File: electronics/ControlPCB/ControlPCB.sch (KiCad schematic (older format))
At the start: 39 parts, among them CON1 12VINPUT, P1 Opto1, P2 Opto2, P3 Opto3, P4 Opto4, P5 Opto5, P6 Opto6, P7 Tool, U1 POLOLU_A4988, U2 POLOLU_A4988, U3 POLOLU_A4988, U4 POLOLU_A4988, U5 POLOLU_A4988, U6 POLOLU_A4988, U7 POLOLU_A4988

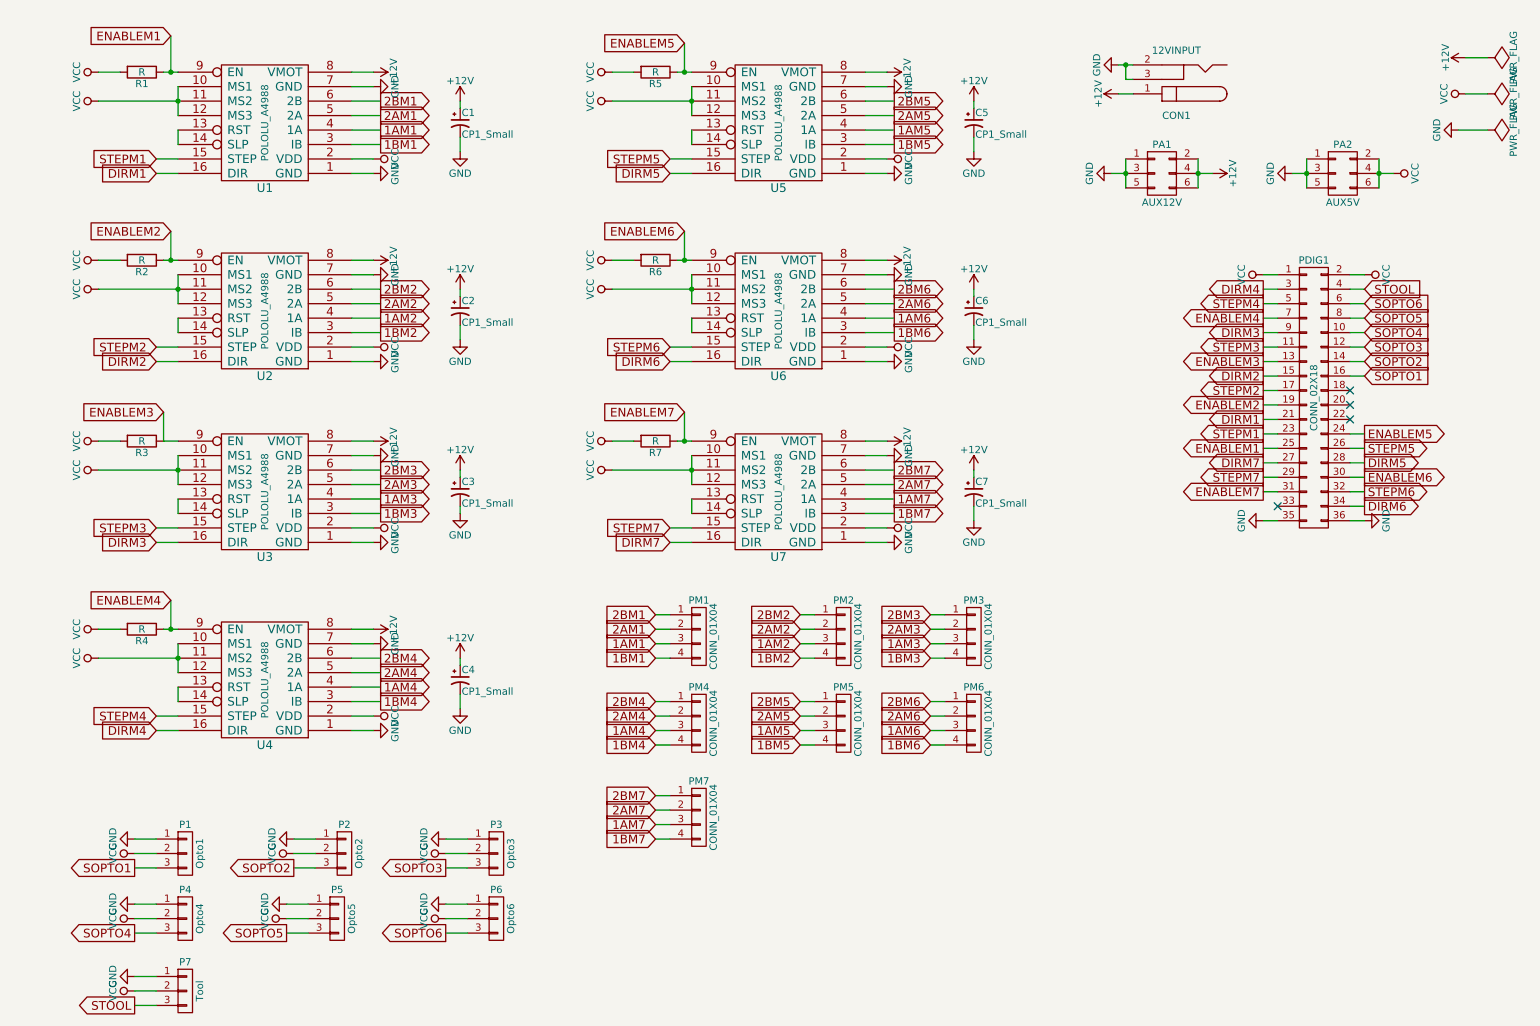
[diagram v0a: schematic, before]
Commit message: changes added
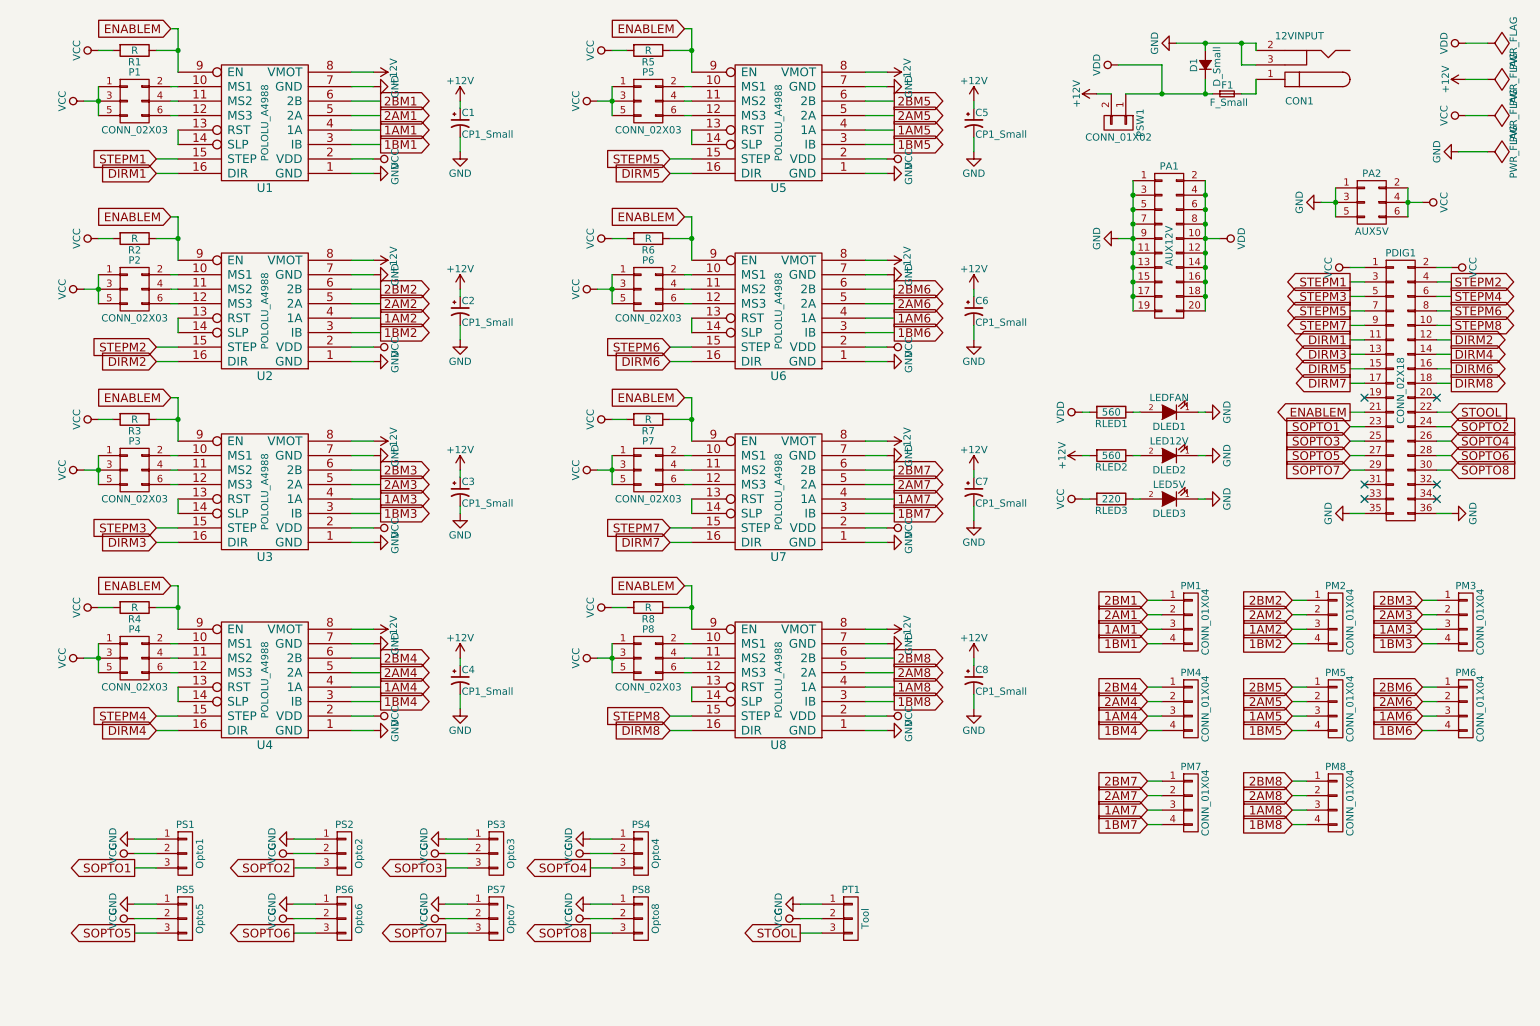
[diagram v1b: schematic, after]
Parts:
- removed PA1: AUX12V, Pin_Headers:Pin_Header_Straight_2x03, symbol CONN_02X03
- added C8: CP1_Small, Capacitors_ThroughHole:C_Radial_D6.3_L11.2_P2.5, symbol CP1_Small
- added D1: D_Small, symbol D_Small
- added DLED1: LEDFAN, symbol LED
- added DLED2: LED12V, symbol LED
- added DLED3: LED5V, symbol LED
- added F1: F_Small, symbol F_Small
- added P1, P2, P3, P4, P5, P6, P7, P8: CONN_02X03, symbol CONN_02X03
- added PA1: AUX12V, symbol CONN_02X10
- added PM8: CONN_01X04, Pin_Headers:Pin_Header_Straight_1x04, symbol CONN_01X04
- added PS7: Opto7, Pin_Headers:Pin_Header_Straight_1x03, symbol CONN_01X03
- added PS8: Opto8, Pin_Headers:Pin_Header_Straight_1x03, symbol CONN_01X03
- added PSW1: CONN_01X02, symbol CONN_01X02
- added R8: R, Resistors_ThroughHole:Resistor_Horizontal_RM7mm, symbol R
- added RLED1, RLED2: 560, symbol R
- added RLED3: 220, symbol R
- added U8: POLOLU_A4988, POL:POLA4988, symbol POLOLU_A4988
- renumbered P1 to PS1, P2 to PS2, P3 to PS3, P4 to PS4, P5 to PS5, P6 to PS6, P7 to PT1
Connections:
- net +12V: now also C8.1, PSW1.2 (P2), RLED2.2, U8.8 (VMOT); no longer CON1.1
- net DIRM1: now also PDIG1.11 (P11); no longer PDIG1.21 (P21)
- net DIRM2: now also PDIG1.12 (P12); no longer PDIG1.15 (P15)
- net DIRM3: now also PDIG1.13 (P13); no longer PDIG1.9 (P9)
- net DIRM4: now also PDIG1.14 (P14); no longer PDIG1.3 (P3)
- net DIRM5: now also PDIG1.15 (P15); no longer PDIG1.28 (P28)
- net DIRM6: now also PDIG1.16 (P16); no longer PDIG1.34 (P34)
- net DIRM7: now also PDIG1.17 (P17); no longer PDIG1.27 (P27)
- net GND: now also C8.2, D1.2 (A), DLED1.1 (K), DLED2.1 (K), DLED3.1 (K), PA1.1 (P1), PA1.11 (P11), PA1.13 (P13), PA1.15 (P15), PA1.17 (P17), PA1.19 (P19), PA1.3 (P3), PA1.5 (P5), PA1.7 (P7), PA1.9 (P9), PS7.1 (P1), PS8.1 (P1), U8.1 (GND), U8.7 (GND)
- net SOPTO1: now also PDIG1.23 (P23); no longer PDIG1.16 (P16)
- net SOPTO2: now also PDIG1.24 (P24); no longer PDIG1.14 (P14)
- net SOPTO3: now also PDIG1.25 (P25); no longer PDIG1.12 (P12)
- net SOPTO4: now also PDIG1.26 (P26); no longer PDIG1.10 (P10)
- net SOPTO5: now also PDIG1.27 (P27); no longer PDIG1.8 (P8)
- net SOPTO6: now also PDIG1.28 (P28); no longer PDIG1.6 (P6)
- net STEPM1: now also PDIG1.3 (P3); no longer PDIG1.23 (P23)
- net STEPM2: now also PDIG1.4 (P4); no longer PDIG1.17 (P17)
- net STEPM3: now also PDIG1.5 (P5); no longer PDIG1.11 (P11)
- net STEPM4: now also PDIG1.6 (P6); no longer PDIG1.5 (P5)
- net STEPM5: now also PDIG1.7 (P7); no longer PDIG1.26 (P26)
- net STEPM6: now also PDIG1.8 (P8); no longer PDIG1.32 (P32)
- net STEPM7: now also PDIG1.9 (P9); no longer PDIG1.29 (P29)
- net STOOL: now also PDIG1.22 (P22); no longer PDIG1.4 (P4)
- net VCC: now also P1.1 (P1), P1.3 (P3), P1.5 (P5), P2.1 (P1), P2.3 (P3), P2.5 (P5), P3.1 (P1), P3.3 (P3), P3.5 (P5), P4.1 (P1), P4.3 (P3), P4.5 (P5), P5.1 (P1), P5.3 (P3), P5.5 (P5), P6.1 (P1), P6.3 (P3), P6.5 (P5), P7.1 (P1), P7.3 (P3), P7.5 (P5), P8.1 (P1), P8.3 (P3), P8.5 (P5), PS7.2 (P2), PS8.2 (P2), R8.2, RLED3.2, U8.2 (VDD); no longer U1.10 (MS1), U1.11 (MS2), U1.12 (MS3), U2.10 (MS1), U2.11 (MS2), U2.12 (MS3), U3.10 (MS1), U3.11 (MS2), U3.12 (MS3), U4.10 (MS1), U4.11 (MS2), U4.12 (MS3), U5.10 (MS1), U5.11 (MS2), U5.12 (MS3), U6.10 (MS1), U6.11 (MS2), U6.12 (MS3), U7.10 (MS1), U7.11 (MS2), U7.12 (MS3)
- net DIRM8: now reaches PDIG1.18 (P18)
- net DIRM8: now also U8.16 (DIR)
- net ENABLEM1 renamed ENABLEM
- net ENABLEM: now also PDIG1.21 (P21), R2.1, R3.1, R4.1, R5.1, R6.1, R7.1, U2.9 (EN), U3.9 (EN), U4.9 (EN), U5.9 (EN), U6.9 (EN), U7.9 (EN), R8.1, U8.9 (EN); no longer PDIG1.25 (P25)
- removed net ENABLEM2: PDIG1.19 (P19), R2.1, U2.9 (EN)
- removed net ENABLEM3: PDIG1.13 (P13), R3.1, U3.9 (EN)
- removed net ENABLEM4: PDIG1.7 (P7), R4.1, U4.9 (EN)
- removed net ENABLEM5: PDIG1.24 (P24), R5.1, U5.9 (EN)
- removed net ENABLEM6: PDIG1.30 (P30), R6.1, U6.9 (EN)
- removed net ENABLEM7: PDIG1.31 (P31), R7.1, U7.9 (EN)
- new net: P1.2 (P2), U1.10 (MS1)
- new net: P1.4 (P4), U1.11 (MS2)
- new net: P1.6 (P6), U1.12 (MS3)
- new net: P2.2 (P2), U2.10 (MS1)
- new net: P2.4 (P4), U2.11 (MS2)
- new net: P2.6 (P6), U2.12 (MS3)
- new net: P3.2 (P2), U3.10 (MS1)
- new net: P3.4 (P4), U3.11 (MS2)
- new net: P3.6 (P6), U3.12 (MS3)
- new net: P4.2 (P2), U4.10 (MS1)
- new net: P4.4 (P4), U4.11 (MS2)
- new net: P4.6 (P6), U4.12 (MS3)
- new net: P5.2 (P2), U5.10 (MS1)
- new net: P5.4 (P4), U5.11 (MS2)
- new net: P5.6 (P6), U5.12 (MS3)
- new net: P6.2 (P2), U6.10 (MS1)
- new net: P6.4 (P4), U6.11 (MS2)
- new net: P6.6 (P6), U6.12 (MS3)
- new net: P7.2 (P2), U7.10 (MS1)
- new net: P7.4 (P4), U7.11 (MS2)
- new net: P7.6 (P6), U7.12 (MS3)
- new net: CON1.1, F1.2
- new net: P8.2 (P2), U8.10 (MS1)
- new net: P8.4 (P4), U8.11 (MS2)
- new net: P8.6 (P6), U8.12 (MS3)
- new net: U8.13 (RST), U8.14 (SLP)
- new net: DLED1.2 (A), RLED1.1
- new net: DLED2.2 (A), RLED2.1
- new net: DLED3.2 (A), RLED3.1
- new net 1AM8: PM8.3 (P3), U8.4 (1A)
- new net 1BM8: PM8.4 (P4), U8.3 (IB)
- new net 2AM8: PM8.2 (P2), U8.5 (2A)
- new net 2BM8: PM8.1 (P1), U8.6 (2B)
- new net SOPTO7: PDIG1.29 (P29), PS7.3 (P3)
- new net SOPTO8: PDIG1.30 (P30), PS8.3 (P3)
- new net STEPM8: PDIG1.10 (P10), U8.15 (STEP)
- new net VDD: D1.1 (K), F1.1, PA1.10 (P10), PA1.12 (P12), PA1.14 (P14), PA1.16 (P16), PA1.18 (P18), PA1.2 (P2), PA1.20 (P20), PA1.4 (P4), PA1.6 (P6), PA1.8 (P8), PSW1.1 (P1), RLED1.2
- no-connect marks 4 -> 6
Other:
- moved on the sheet: CON1, PA2, PDIG1, PM1, PM2, PM3, PM4, PM5, PM6, PM7, PS4, PS5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

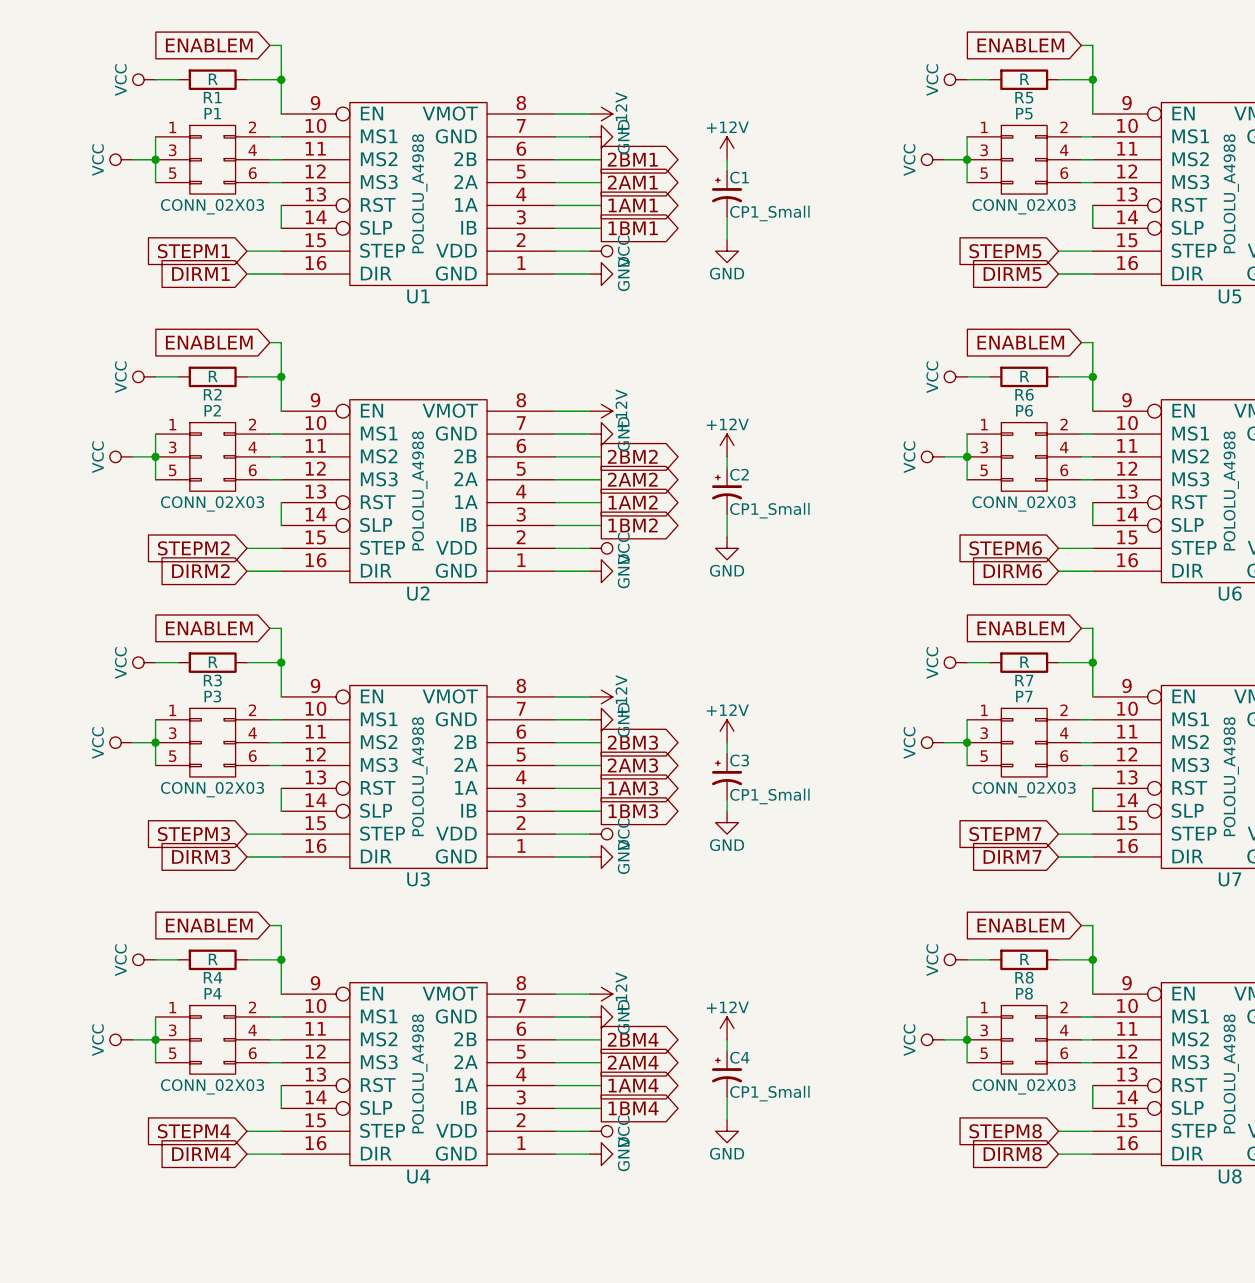
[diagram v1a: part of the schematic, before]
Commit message: PCB update
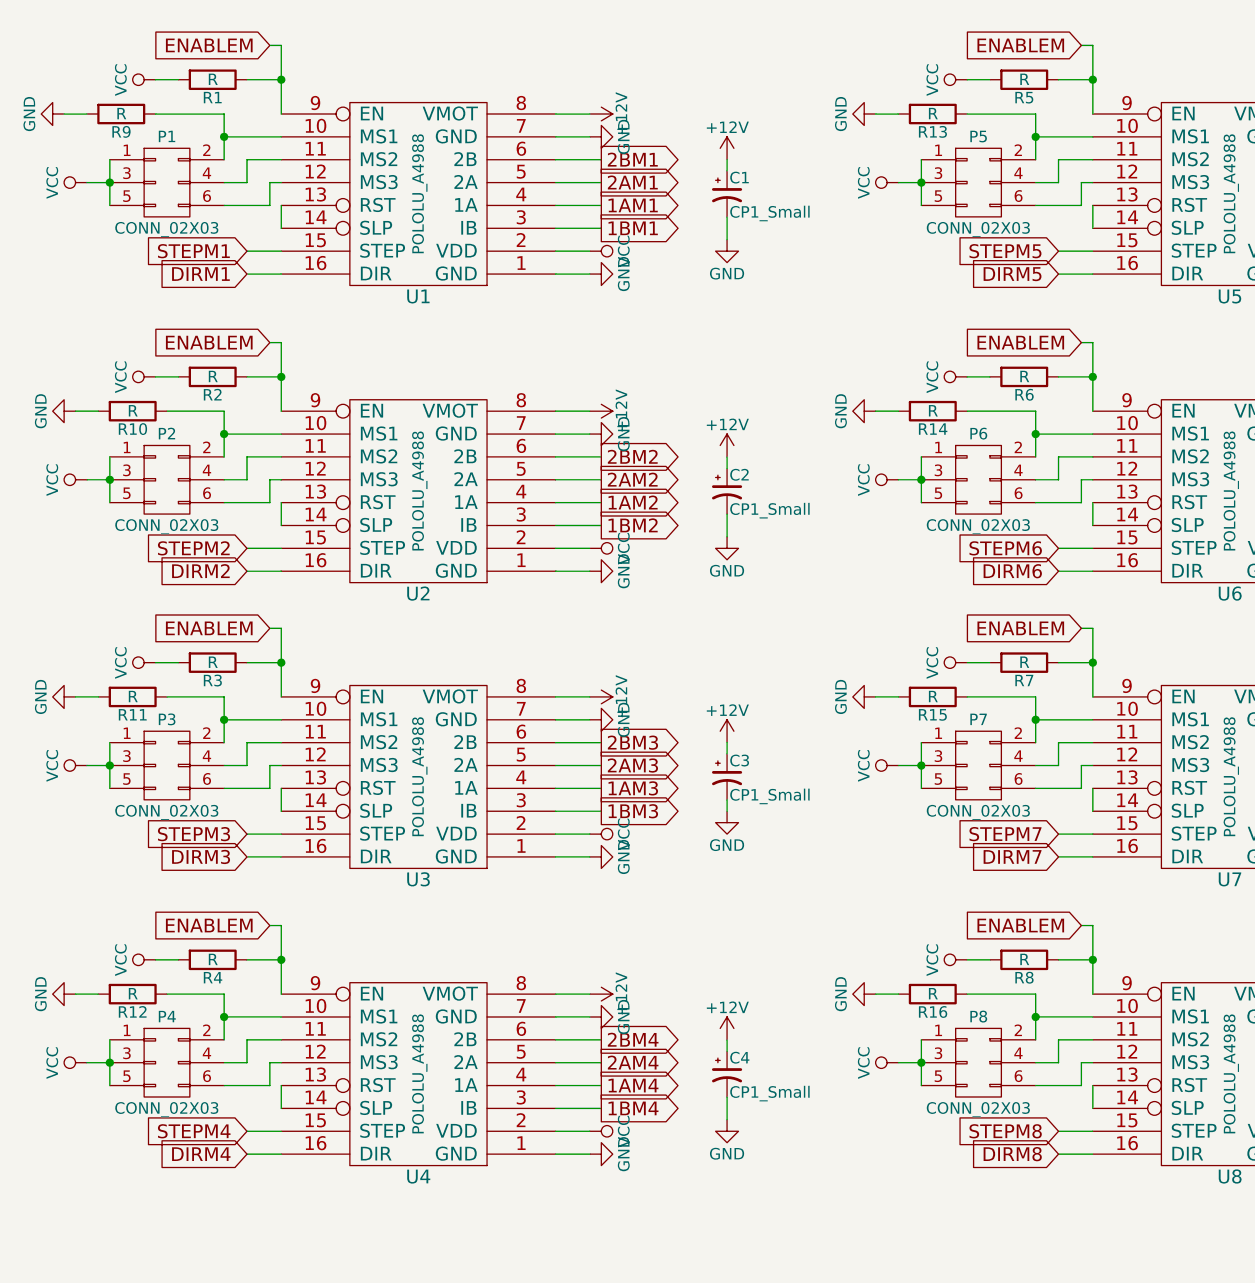
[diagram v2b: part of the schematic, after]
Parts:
- added R10, R11, R12, R13, R14, R15, R16, R9: R, Resistors_SMD:R_1206_HandSoldering, symbol R
- C1, C2, C3, C4, C5, C6, C7, C8: footprint Capacitors_ThroughHole:C_Radial_D6.3_L11.2_P2.5 -> Capacitors_SMD:c_elec_6.3x5.7
- D1: footprint (none) -> Diodes_ThroughHole:Diode_DO-35_SOD27_Horizontal_RM10
- DLED1, DLED2, DLED3: footprint (none) -> LEDs:LED_1206
- F1: footprint (none) -> Fuse_Holders_and_Fuses:BladeFuse-CarType
- P1, P2, P3, P4, P5, P6, P7, P8: footprint (none) -> Pin_Headers:Pin_Header_Straight_2x03
- PA1: footprint (none) -> Pin_Headers:Pin_Header_Straight_2x10
- PSW1: footprint (none) -> Pin_Headers:Pin_Header_Straight_1x02
- R1, R2, R3, R4, R5, R6, R7, R8: footprint Resistors_ThroughHole:Resistor_Horizontal_RM7mm -> Resistors_SMD:R_1206_HandSoldering
- RLED1, RLED2, RLED3: footprint (none) -> Resistors_SMD:R_1206_HandSoldering
- U1, U2, U3, U4, U5, U6, U7, U8: footprint POL:POLA4988 -> Pololu:SWDIP8_.6W
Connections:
- net GND: now also R10.2, R11.2, R12.2, R13.2, R14.2, R15.2, R16.2, R9.2
- net at P1.2 (P2), U1.10 (MS1): now also R9.1
- net at P2.2 (P2), U2.10 (MS1): now also R10.1
- net at P3.2 (P2), U3.10 (MS1): now also R11.1
- net at P4.2 (P2), U4.10 (MS1): now also R12.1
- net at P5.2 (P2), U5.10 (MS1): now also R13.1
- net at P6.2 (P2), U6.10 (MS1): now also R14.1
- net at P7.2 (P2), U7.10 (MS1): now also R15.1
- net at P8.2 (P2), U8.10 (MS1): now also R16.1
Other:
- moved on the sheet: P1, P2, P3, P4, P5, P6, P7, P8
